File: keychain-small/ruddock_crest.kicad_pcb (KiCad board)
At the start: 2 copper layers, 38.1 x 45.7 mm, 4 parts

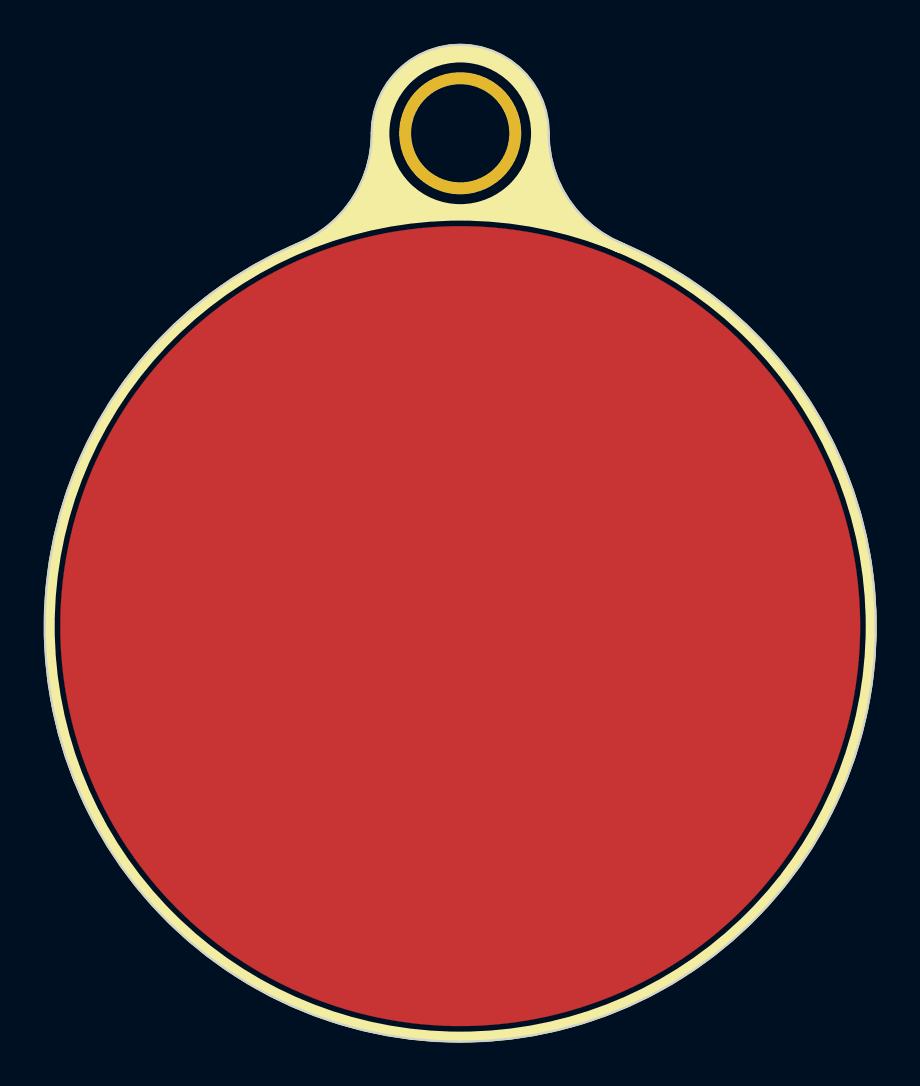
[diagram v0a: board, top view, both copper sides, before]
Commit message: Migrate to KiCad 5.1.4
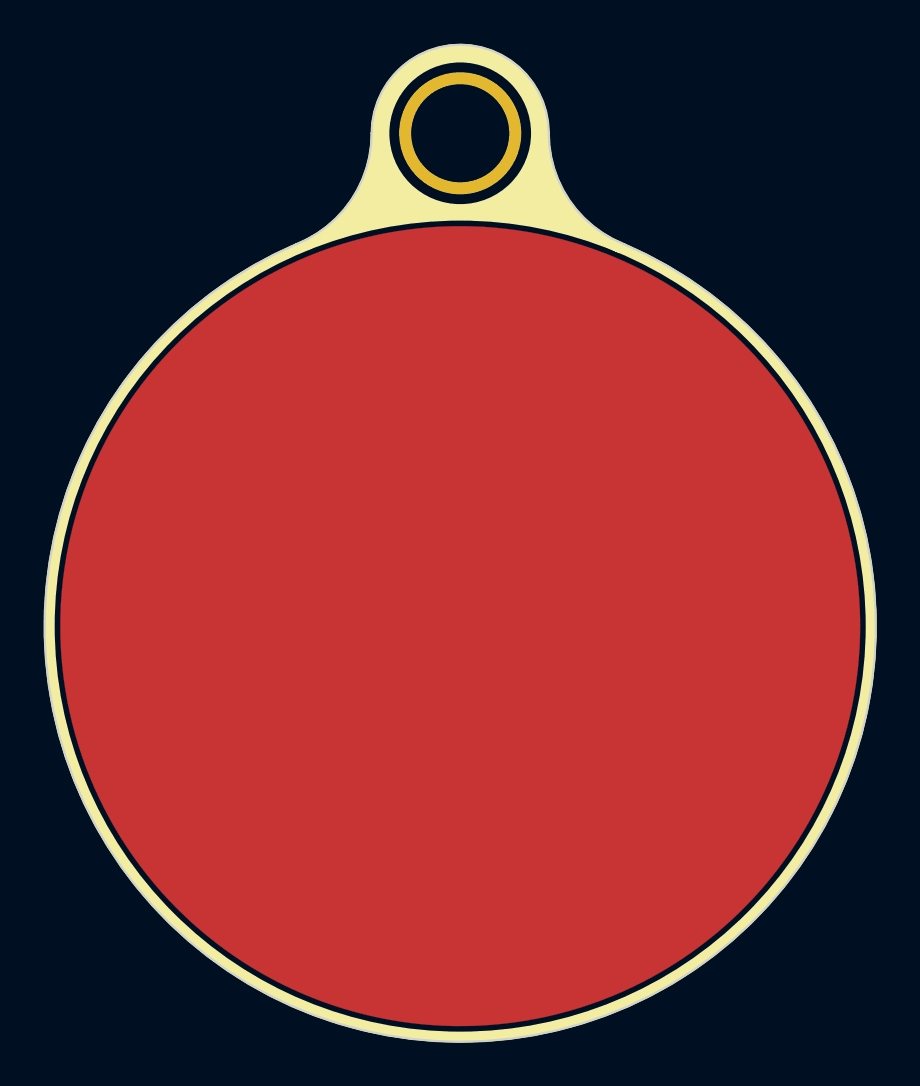
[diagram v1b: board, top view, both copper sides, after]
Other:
- outline, holes or cut-outs redrawn
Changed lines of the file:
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@@
-(kicad_pcb (version 20171130) (host pcbnew "(5.0.1)-3")
+(kicad_pcb (version 20171130) (host pcbnew "(5.1.4)-1")
   (general
     (thickness 1.6)
@@
     (zone_45_only no)
     (trace_min 0.2)
-    (segment_width 0.5)
-    (edge_width 0.1)
     (via_size 0.8)
     (via_drill 0.4)
@@
     (uvia_min_size 0.2)
     (uvia_min_drill 0.1)
+    (edge_width 0.1)
+    (segment_width 0.5)
     (pcb_text_width 0.3)
     (pcb_text_size 1.5 1.5)
@@
       (xy 0.287869 -18.341347)) (layer F.Cu) (width 0.01))
   )
+  (gr_arc (start 140.97 107.95) (end 133.466674 90.423999) (angle -313.6458442) (layer Edge.Cuts) (width 0.1))
   (gr_arc (start 150.510695 85.344) (end 148.300896 90.576399) (angle 67.1) (layer B.SilkS) (width 0.5))
   (gr_arc (start 150.495 85.344) (end 148.285201 90.576399) (angle 67.1) (layer F.SilkS) (width 0.5))
@@
   (gr_arc (start 131.445 85.344) (end 133.984999 90.423999) (angle -63.4) (layer B.SilkS) (width 0.5))
   (gr_arc (start 131.445 85.344) (end 133.984999 90.423999) (angle -63.4) (layer F.SilkS) (width 0.5))
-  (gr_arc (start 140.97 107.95) (end 133.477001 90.424001) (angle -313.703074) (layer Edge.Cuts) (width 0.1))
-  (gr_arc (start 150.495 85.344) (end 148.463001 90.423999) (angle 68.2) (layer Edge.Cuts) (width 0.1))
+  (gr_arc (start 150.505326 85.344134) (end 148.473327 90.424133) (angle 68.2) (layer Edge.Cuts) (width 0.1))
   (gr_circle (center 150.495 85.344) (end 150.368 85.344) (layer Dwgs.User) (width 0.1))
   (gr_circle (center 150.495 85.344) (end 145.034 85.344) (layer Dwgs.User) (width 0.1))
-  (gr_arc (start 131.445 85.344) (end 133.476999 90.423999) (angle -68.19859051) (layer Edge.Cuts) (width 0.1))
+  (gr_arc (start 131.434674 85.343999) (end 133.466673 90.423998) (angle -68.19859051) (layer Edge.Cuts) (width 0.1))
   (gr_circle (center 131.445 85.344) (end 131.572 85.344) (layer Dwgs.User) (width 0.1))
   (gr_circle (center 131.445 85.344) (end 136.906 85.344) (layer Dwgs.User) (width 0.1))
